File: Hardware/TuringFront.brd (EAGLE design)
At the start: 107 x 49.5 mm, 73 parts, among them T1 2N3904, U1 TL074_

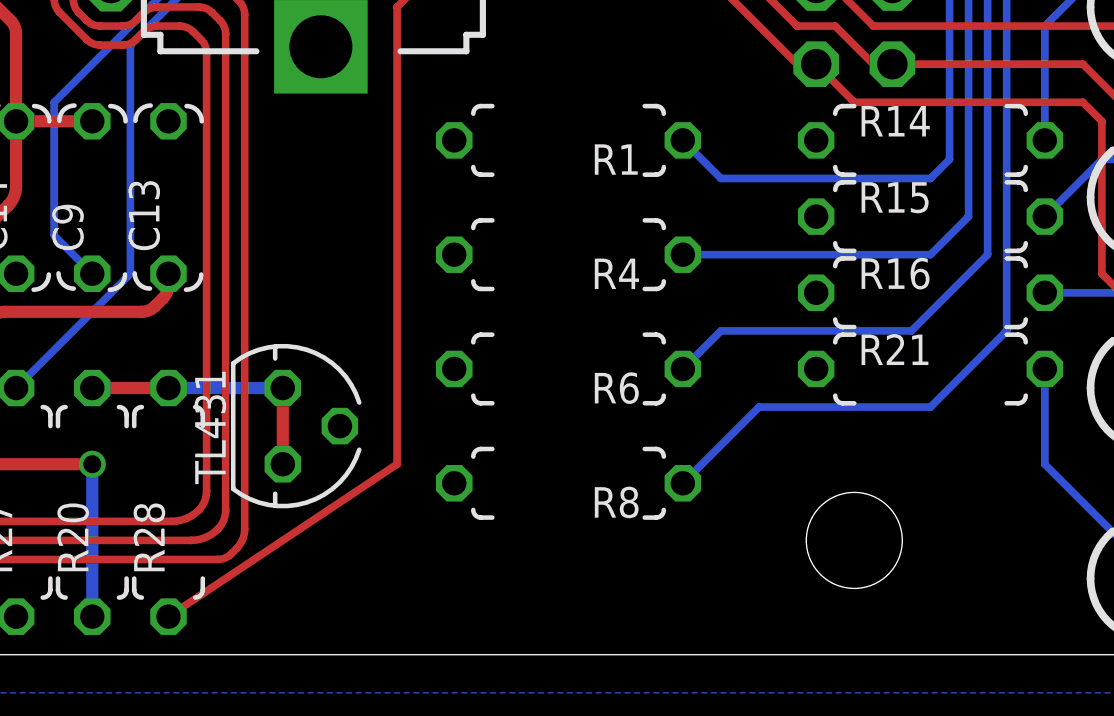
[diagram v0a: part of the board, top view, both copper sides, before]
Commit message: Finalised V4 PCBs
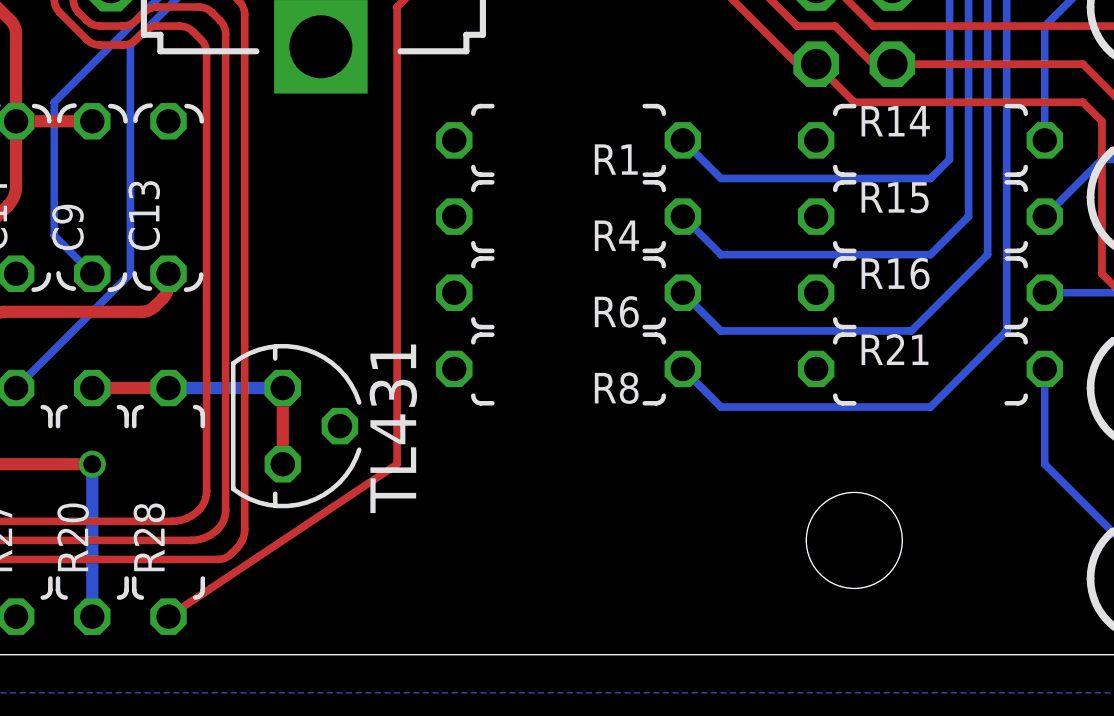
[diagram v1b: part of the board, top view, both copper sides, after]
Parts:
- moved R8 3.81 mm to (85.7, 9.53)
- moved R6 2.54 mm to (85.7, 12.1)
- moved R4 1.27 mm to (85.7, 14.6)
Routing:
- net N$31: track 40.5 -> 41.0 mm
- net N$33: track 35.4 -> 34.9 mm
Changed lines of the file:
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@@
 <layer number="19" name="Unrouted" color="6" fill="1" visible="no" active="yes"/>
 <layer number="20" name="Dimension" color="15" fill="1" visible="yes" active="yes"/>
-<layer number="21" name="tPlace" color="7" fill="1" visible="no" active="yes"/>
-<layer number="22" name="bPlace" color="7" fill="1" visible="yes" active="yes"/>
+<layer number="21" name="tPlace" color="7" fill="1" visible="yes" active="yes"/>
+<layer number="22" name="bPlace" color="7" fill="1" visible="no" active="yes"/>
 <layer number="23" name="tOrigins" color="15" fill="1" visible="yes" active="yes"/>
-<layer number="24" name="bOrigins" color="15" fill="1" visible="yes" active="yes"/>
-<layer number="25" name="tNames" color="7" fill="1" visible="no" active="yes"/>
-<layer number="26" name="bNames" color="7" fill="1" visible="yes" active="yes"/>
-<layer number="27" name="tValues" color="7" fill="1" visible="no" active="yes"/>
+<layer number="24" name="bOrigins" color="15" fill="1" visible="no" active="yes"/>
+<layer number="25" name="tNames" color="7" fill="1" visible="yes" active="yes"/>
+<layer number="26" name="bNames" color="7" fill="1" visible="no" active="yes"/>
+<layer number="27" name="tValues" color="7" fill="1" visible="yes" active="yes"/>
 <layer number="28" name="bValues" color="7" fill="1" visible="yes" active="yes"/>
 <layer number="29" name="tStop" color="7" fill="3" visible="no" active="yes"/>
@@
 <element name="SCALE" library="MusicThingModular" package="9MM_SNAP-IN_POT" value="50k" x="22.86" y="6.35" locked="yes" rot="R270"/>
 <element name="C17" library="TomW" package="C050-024X044" value="1n" x="64.77" y="15.24" rot="R90"/>
-<element name="TL431" library="TomW" package="TO92-CLP" value="" x="76.2" y="7.62" rot="R270"/>
+<element name="TL431" library="TomW" package="TO92-CLP" value="" x="76.2" y="7.62" smashed="yes" rot="R270">
+<attribute name="NAME" x="80.645" y="7.62" size="1.524" layer="25" ratio="10" rot="R270" align="top-center"/>
+</element>
 <element name="R20" library="TomW" package="0207/7" value="3.3k" x="69.85" y="5.08" rot="R90"/>
 <element name="C18" library="rcl" package="C050-035X075" value="0.47uf" x="49.53" y="15.24" rot="R90"/>
@@
 </element>
 <element name="R1" library="TomW" package="0207/7" value="2.2k" x="85.725" y="17.145" rot="R180"/>
-<element name="R4" library="TomW" package="0207/7" value="2.2k" x="85.725" y="13.335" rot="R180"/>
-<element name="R6" library="TomW" package="0207/7" value="2.2k" x="85.725" y="9.525" rot="R180"/>
-<element name="R8" library="TomW" package="0207/7" value="2.2k" x="85.725" y="5.715" rot="R180"/>
+<element name="R4" library="TomW" package="0207/7" value="2.2k" x="85.725" y="14.605" rot="R180"/>
+<element name="R6" library="TomW" package="0207/7" value="2.2k" x="85.725" y="12.065" rot="R180"/>
+<element name="R8" library="TomW" package="0207/7" value="2.2k" x="85.725" y="9.525" rot="R180"/>
 <element name="R14" library="TomW" package="0207/7" value="2.2k" x="97.79" y="17.145"/>
 <element name="R15" library="TomW" package="0207/7" value="2.2k" x="97.79" y="14.605"/>
@@
 <wire x1="99.06" y1="34.29" x2="99.06" y2="14.605" width="0.254" layer="16"/>
 <wire x1="99.06" y1="14.605" x2="97.79" y2="13.335" width="0.254" layer="16"/>
-<wire x1="97.79" y1="13.335" x2="89.535" y2="13.335" width="0.254" layer="16"/>
+<wire x1="97.79" y1="13.335" x2="90.805" y2="13.335" width="0.254" layer="16"/>
+<wire x1="90.805" y1="13.335" x2="89.535" y2="14.605" width="0.254" layer="16"/>
 </signal>
 <signal name="N$32">
@@
 <wire x1="99.695" y1="13.335" x2="97.155" y2="10.795" width="0.254" layer="16"/>
 <wire x1="97.155" y1="10.795" x2="90.805" y2="10.795" width="0.254" layer="16"/>
-<wire x1="90.805" y1="10.795" x2="89.535" y2="9.525" width="0.254" layer="16"/>
+<wire x1="90.805" y1="10.795" x2="89.535" y2="12.065" width="0.254" layer="16"/>
 </signal>
 <signal name="N$33">
@@
 <wire x1="100.33" y1="27.94" x2="100.33" y2="10.795" width="0.254" layer="16"/>
 <wire x1="100.33" y1="10.795" x2="97.79" y2="8.255" width="0.254" layer="16"/>
-<wire x1="97.79" y1="8.255" x2="92.075" y2="8.255" width="0.254" layer="16"/>
-<wire x1="92.075" y1="8.255" x2="89.535" y2="5.715" width="0.254" layer="16"/>
+<wire x1="97.79" y1="8.255" x2="90.805" y2="8.255" width="0.254" layer="16"/>
+<wire x1="90.805" y1="8.255" x2="89.535" y2="9.525" width="0.254" layer="16"/>
 </signal>
 <signal name="N$34">
@@
 <contactref element="U1" pad="10"/>
 <contactref element="R9" pad="1"/>
-<contactref element="U1" pad="3"/>
 <contactref element="CV_OUT" pad="P$3_SLEEVE"/>
 <contactref element="R12" pad="2"/>
@@
 <vertex x="-1.27" y="50.8"/>
 </polygon>
+<contactref element="U1" pad="3"/>
+<wire x1="93.98" y1="12.065" x2="93.98" y2="9.525" width="0" layer="19" extent="1-1"/>
+<wire x1="93.98" y1="14.605" x2="93.98" y2="12.065" width="0" layer="19" extent="1-1"/>
+<wire x1="93.98" y1="17.145" x2="93.98" y2="14.605" width="0" layer="19" extent="1-1"/>
 </signal>
 <signal name="WRITE_SW_FRONT">
